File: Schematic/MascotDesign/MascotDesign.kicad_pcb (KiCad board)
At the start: 2 copper layers, 64 x 35.6 mm, 42 parts, among them J1 Charger input, J10 AudioJack4, J11 Main power cutoff (soldered s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, J2 PI power USB, J3 LCD LED Power, J4 Dummy Header, J5 Audio in, J6 Audio in, J8 Potentiometer, J9 Speaker 8R, U1 Generic_Buck_Regulator, U2 Generic_Buck_Regulator, U3 TPA3116D2DAD

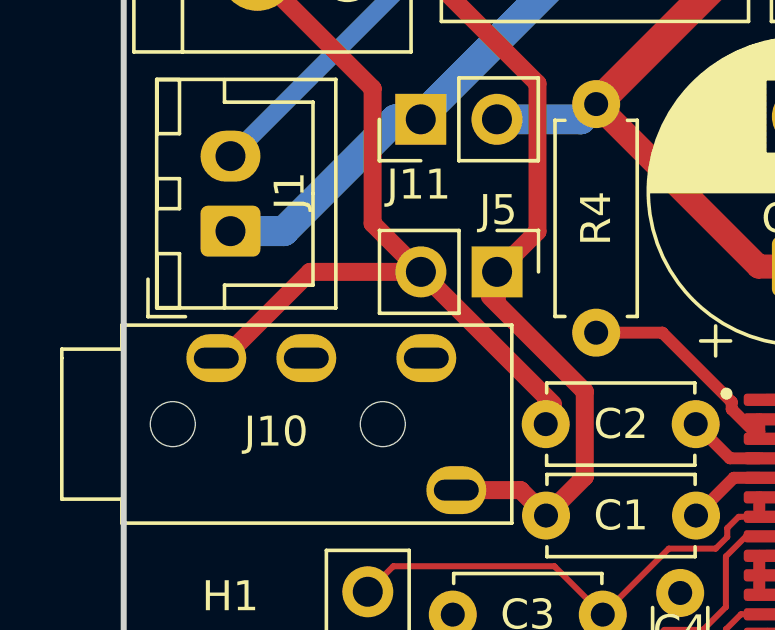
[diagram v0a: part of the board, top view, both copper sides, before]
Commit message: Merge branch 'main' of https://github.com/DrGlaucous/mascot-head-sr-design
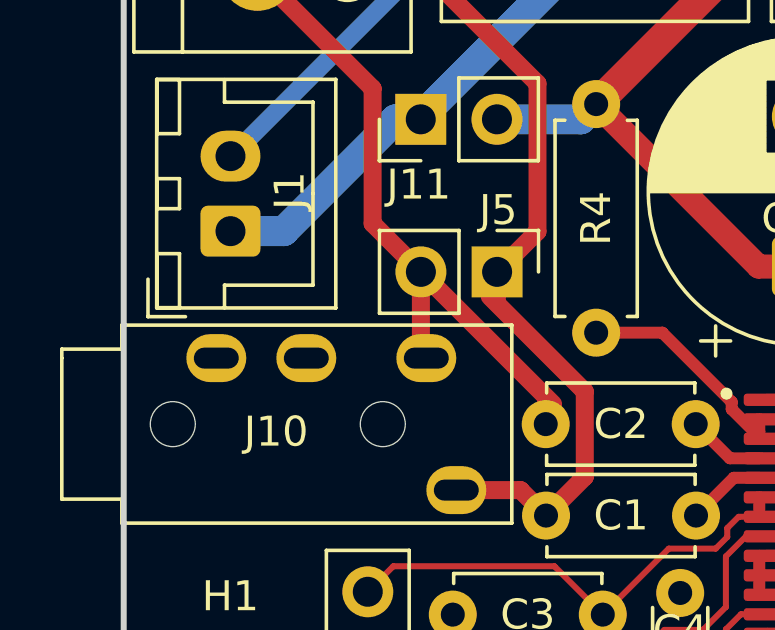
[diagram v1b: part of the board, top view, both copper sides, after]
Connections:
- J10 pad S: Net-(J5-Pin_2) -> Net-(J5-Pin_1)
- J10 pad T: Net-(J5-Pin_1) -> Net-(J5-Pin_2)
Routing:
- net Net-(J5-Pin_2): track 26.9 -> 22.1 mm
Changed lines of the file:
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@@
 		)
 		(pad "R1" thru_hole oval
-			(at 12.15 0)
+			(at 8.15 0)
 			(size 2 1.6)
 			(drill oval 1.5 0.7)
@@
 		)
 		(pad "R2" thru_hole oval
-			(at 8.15 0)
+			(at 5.15 0)
 			(size 2 1.6)
 			(drill oval 1.5 0.7)
@@
 		)
 		(pad "S" thru_hole oval
-			(at 5.15 0)
+			(at 13.15 4.4)
 			(size 2 1.6)
 			(drill oval 1.5 0.7)
 			(layers "*.Cu" "*.Mask")
 			(remove_unused_layers no)
-			(net 4 "Net-(J5-Pin_2)")
+			(net 1 "Net-(J5-Pin_1)")
 			(pintype "passive")
 		)
 		(pad "T" thru_hole oval
-			(at 13.15 4.4)
+			(at 12.15 0)
 			(size 2 1.6)
 			(drill oval 1.5 0.7)
 			(layers "*.Cu" "*.Mask")
 			(remove_unused_layers no)
-			(net 1 "Net-(J5-Pin_1)")
+			(net 4 "Net-(J5-Pin_2)")
 			(pintype "passive")
 		)
@@
 	)
 	(segment
-		(start 80.549 82.382)
-		(end 83.424 79.507)
+		(start 87.122 82.202)
+		(end 87.302 82.382)
 		(width 0.6)
 		(layer "F.Cu")
@@
 	(segment
 		(start 87.122 79.507)
-		(end 91.530248 83.915248)
+		(end 87.122 82.202)
 		(width 0.6)
 		(layer "F.Cu")
@@
 	)
 	(segment
-		(start 91.283248 83.915248)
-		(end 91.283248 84.582)
+		(start 87.122 79.507)
+		(end 91.530248 83.915248)
 		(width 0.6)
 		(layer "F.Cu")
@@
 	)
 	(segment
-		(start 83.424 79.507)
-		(end 87.122 79.507)
+		(start 91.283248 83.915248)
+		(end 91.283248 84.582)
 		(width 0.6)
 		(layer "F.Cu")
